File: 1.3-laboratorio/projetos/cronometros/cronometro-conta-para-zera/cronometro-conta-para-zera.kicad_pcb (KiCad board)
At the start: 2 copper layers, 118.1 x 85.1 mm, 72 parts, among them J1 Barrel_Jack_Switch, SW1 SW_Push, SW2 SW_Push, U1 LM555, U10 CD4511BNSR, U11 HDSP-7803, U12 HDSP-7803, U13 HDSP-7803, U14 HDSP-7803, U2 74HC4518, U3 74HC4518, U4 CD4093, U5 CD4093, U6 74HC73, U7 CD4511BNSR, U8 CD4511BNSR, U9 CD4511BNSR

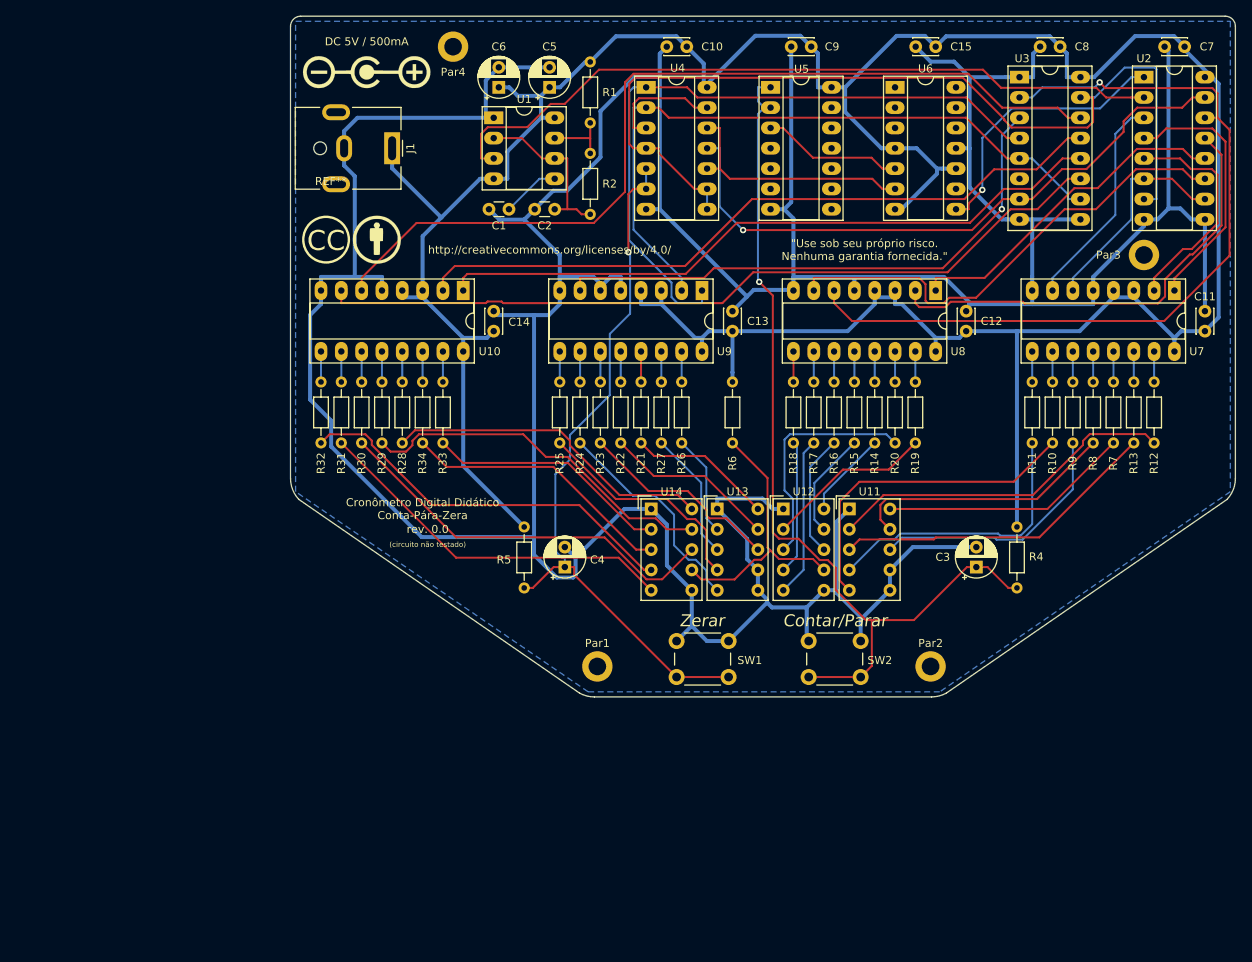
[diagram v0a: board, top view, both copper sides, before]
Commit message: Projeto concluído do Cronômetro Digital Didático Conta-Pára-Zera.
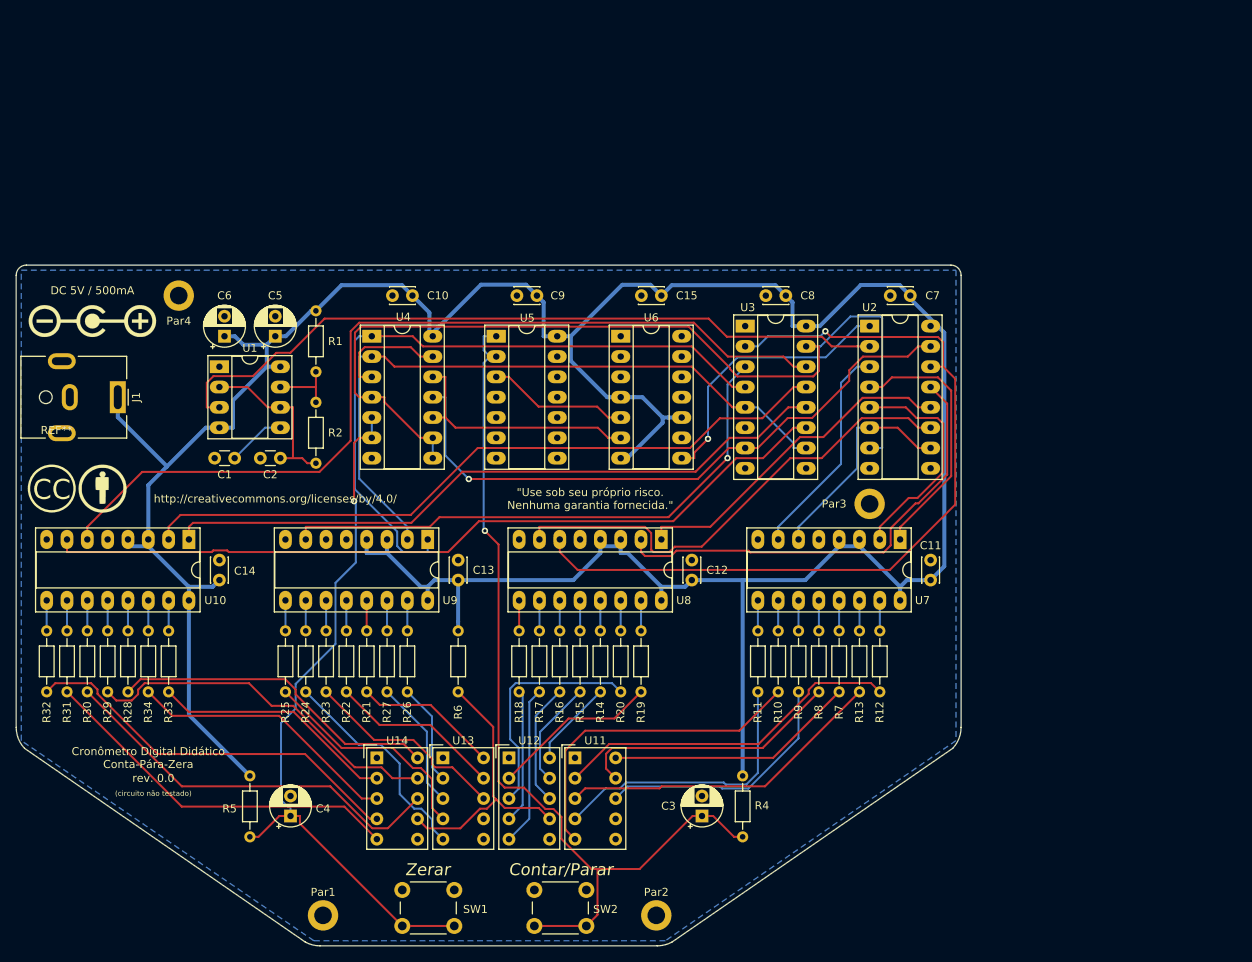
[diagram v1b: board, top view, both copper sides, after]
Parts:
- moved Par1 46.3 mm to (131.1, 136.5)
- moved R4 46.3 mm to (183.5, 119.1)
- moved U14 46.3 mm to (137.8, 116.8)
- moved Par3 46.3 mm to (199.4, 85.1)
- moved U2 46.3 mm to (199.4, 62.9)
- moved U3 46.3 mm to (183.8, 62.9)
- moved C11 46.3 mm to (207.0, 94.6)
- moved C12 46.3 mm to (177.2, 94.6)
- moved C15 46.3 mm to (173.4, 59.1)
- moved R11 46.3 mm to (185.4, 108.6)
- moved R15 46.3 mm to (163.2, 108.6)
- moved R18 46.3 mm to (155.6, 108.6)
- moved R23 46.3 mm to (131.4, 108.6)
- moved R26 46.3 mm to (141.6, 108.6)
- moved R5 46.3 mm to (121.9, 119.1)
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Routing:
- net Earth: track 576.7 -> 0.00 mm
